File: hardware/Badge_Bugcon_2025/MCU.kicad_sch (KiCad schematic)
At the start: 62 parts, among them J1 Conn_01x21, J13 ETH, J14 +1V8, J5 3V3, J8 3V3, SW2 SW_Push, SW3 SW_Push, U6 W25N02KVZEIR, Y1 Crystal, Y2 24MHz

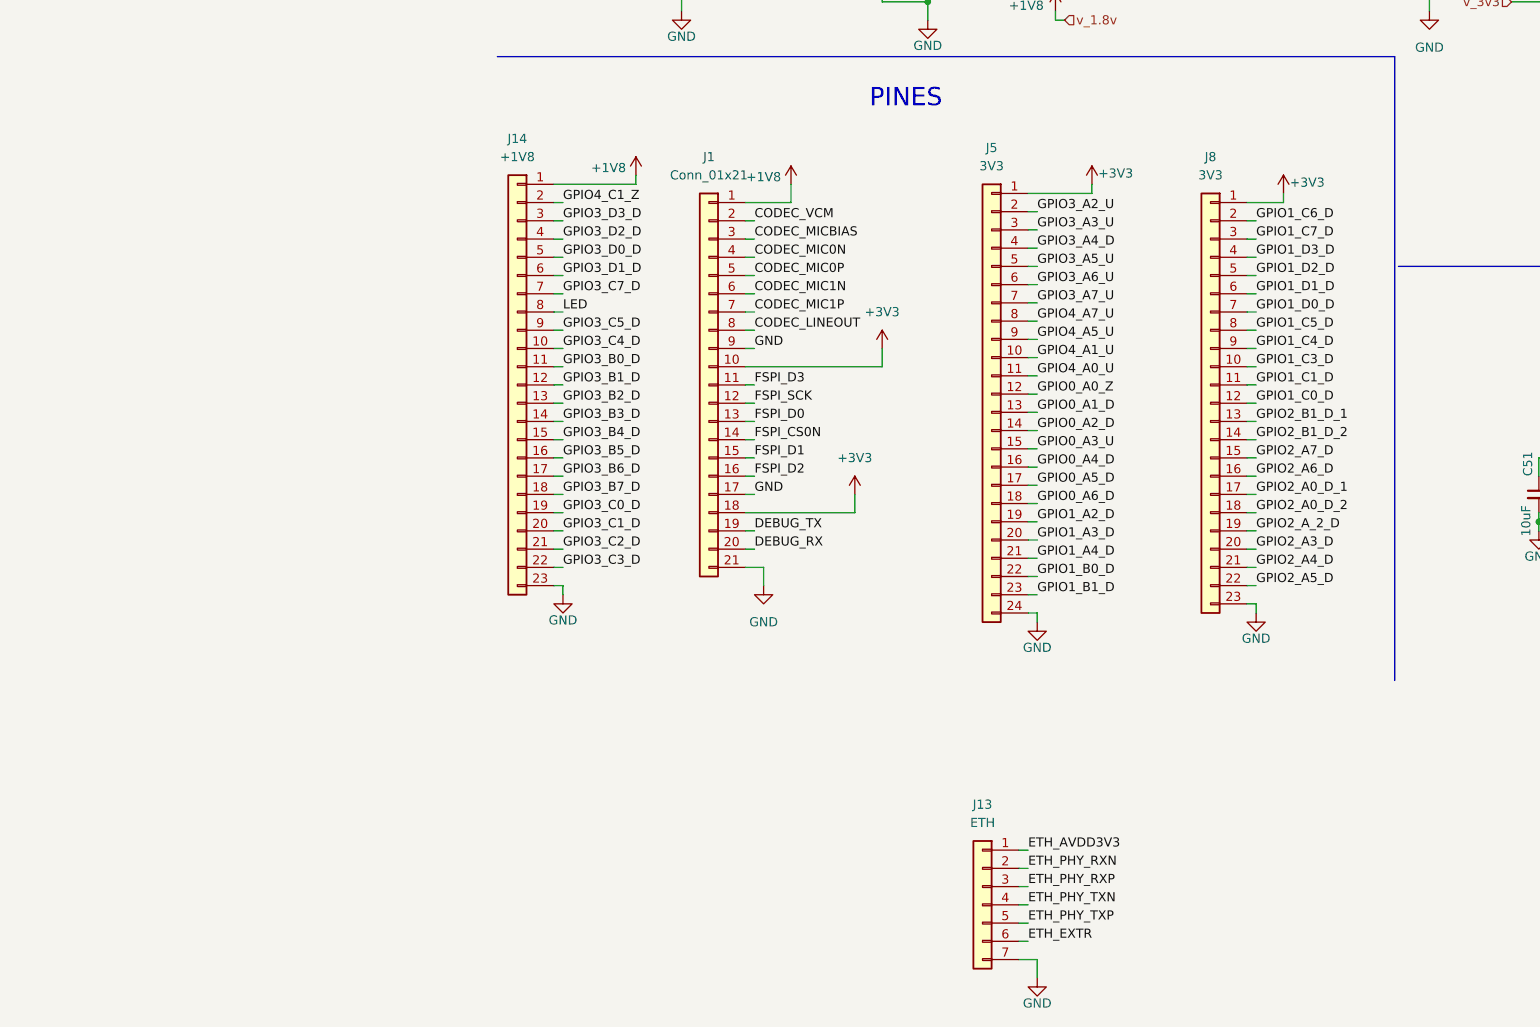
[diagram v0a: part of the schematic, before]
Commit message: feat(Hw):Update_Route
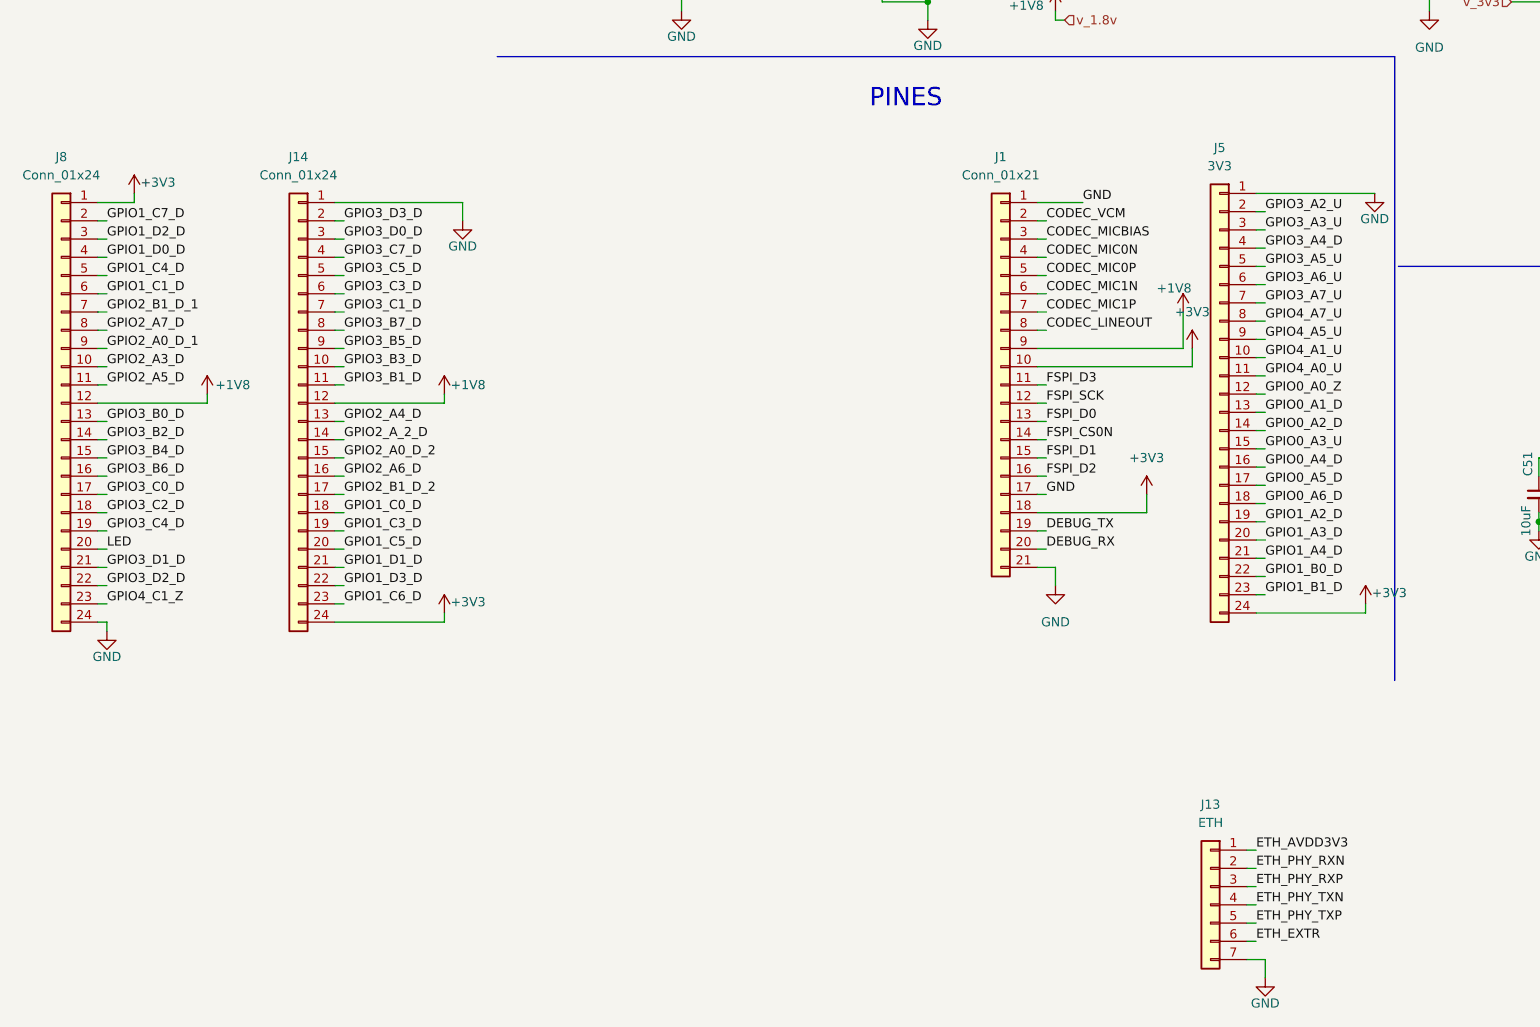
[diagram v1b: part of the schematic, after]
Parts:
- removed J14: +1V8, Connector_PinHeader_2.54mm:PinHeader_1x23_P2.54mm_Vertical, symbol Connector_Generic:Conn_01x23
- removed J8: 3V3, Connector_PinSocket_2.54mm:PinSocket_1x23_P2.54mm_Vertical, symbol Connector_Generic:Conn_01x23
- added J14, J8: Conn_01x24, Connector_PinSocket_2.54mm:PinSocket_1x24_P2.54mm_Vertical, symbol Connector_Generic:Conn_01x24
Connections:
- net +1V8: now also J1.9 (Pin_9), J14.12 (Pin_12), J8.12 (Pin_12); no longer J1.1 (Pin_1)
- net +3V3: now also J5.24 (Pin_24), J14.24 (Pin_24), J8.1 (Pin_1); no longer J5.1 (Pin_1)
- net GND: now also J1.1 (Pin_1), J5.1 (Pin_1), J14.1 (Pin_1), J8.24 (Pin_24); no longer J1.9 (Pin_9), J5.24 (Pin_24)
- net GPIO1_C0_D: now also J14.18 (Pin_18)
- net GPIO1_C1_D: now also J8.6 (Pin_6)
- net GPIO1_C3_D: now also J14.19 (Pin_19)
- net GPIO1_C4_D: now also J8.5 (Pin_5)
- net GPIO1_C5_D: now also J14.20 (Pin_20)
- net GPIO1_C6_D: now also J14.23 (Pin_23)
- net GPIO1_C7_D: now also J8.2 (Pin_2)
- net GPIO1_D0_D: now also J8.4 (Pin_4)
- net GPIO1_D1_D: now also J14.21 (Pin_21)
- net GPIO1_D2_D: now also J8.3 (Pin_3)
- net GPIO1_D3_D: now also J14.22 (Pin_22)
- net GPIO2_A0_D_1: now also J8.9 (Pin_9)
- net GPIO2_A0_D_2: now also J14.15 (Pin_15)
- net GPIO2_A3_D: now also J8.10 (Pin_10)
- net GPIO2_A4_D: now also J14.13 (Pin_13)
- net GPIO2_A5_D: now also J8.11 (Pin_11)
- net GPIO2_A6_D: now also J14.16 (Pin_16)
- net GPIO2_A7_D: now also J8.8 (Pin_8)
- net GPIO2_A_2_D: now also J14.14 (Pin_14)
- net GPIO2_B1_D_1: now also J8.7 (Pin_7)
- net GPIO2_B1_D_2: now also J14.17 (Pin_17)
- net GPIO3_B0_D: now also J8.13 (Pin_13)
- net GPIO3_B1_D: now also J14.11 (Pin_11)
- net GPIO3_B2_D: now also J8.14 (Pin_14)
- net GPIO3_B3_D: now also J14.10 (Pin_10)
- net GPIO3_B4_D: now also J8.15 (Pin_15)
- net GPIO3_B5_D: now also J14.9 (Pin_9)
- net GPIO3_B6_D: now also J8.16 (Pin_16)
- net GPIO3_B7_D: now also J14.8 (Pin_8)
- net GPIO3_C0_D: now also J8.17 (Pin_17)
- net GPIO3_C1_D: now also J14.7 (Pin_7)
- net GPIO3_C2_D: now also J8.18 (Pin_18)
- net GPIO3_C3_D: now also J14.6 (Pin_6)
- net GPIO3_C4_D: now also J8.19 (Pin_19)
- net GPIO3_C5_D: now also J14.5 (Pin_5)
- net GPIO3_C7_D: now also J14.4 (Pin_4)
- net GPIO3_D0_D: now also J14.3 (Pin_3)
- net GPIO3_D1_D: now also J8.21 (Pin_21)
- net GPIO3_D2_D: now also J8.22 (Pin_22)
- net GPIO3_D3_D: now also J14.2 (Pin_2)
- net GPIO4_C1_Z: now also J8.23 (Pin_23)
- net LED: now also J8.20 (Pin_20)
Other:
- moved on the sheet: J1, J13, J5
